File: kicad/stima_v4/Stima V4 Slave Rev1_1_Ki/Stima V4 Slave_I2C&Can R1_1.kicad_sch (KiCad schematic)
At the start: 45 parts, among them J2 6P, J3 3P, U4 TJA1443ATK, U5 NM PCA9616PW, U6 PCA9517D (TCA9517D), U7 ST732M50R, U8 AP22653QW6-7, U9 AP22653QW6-7

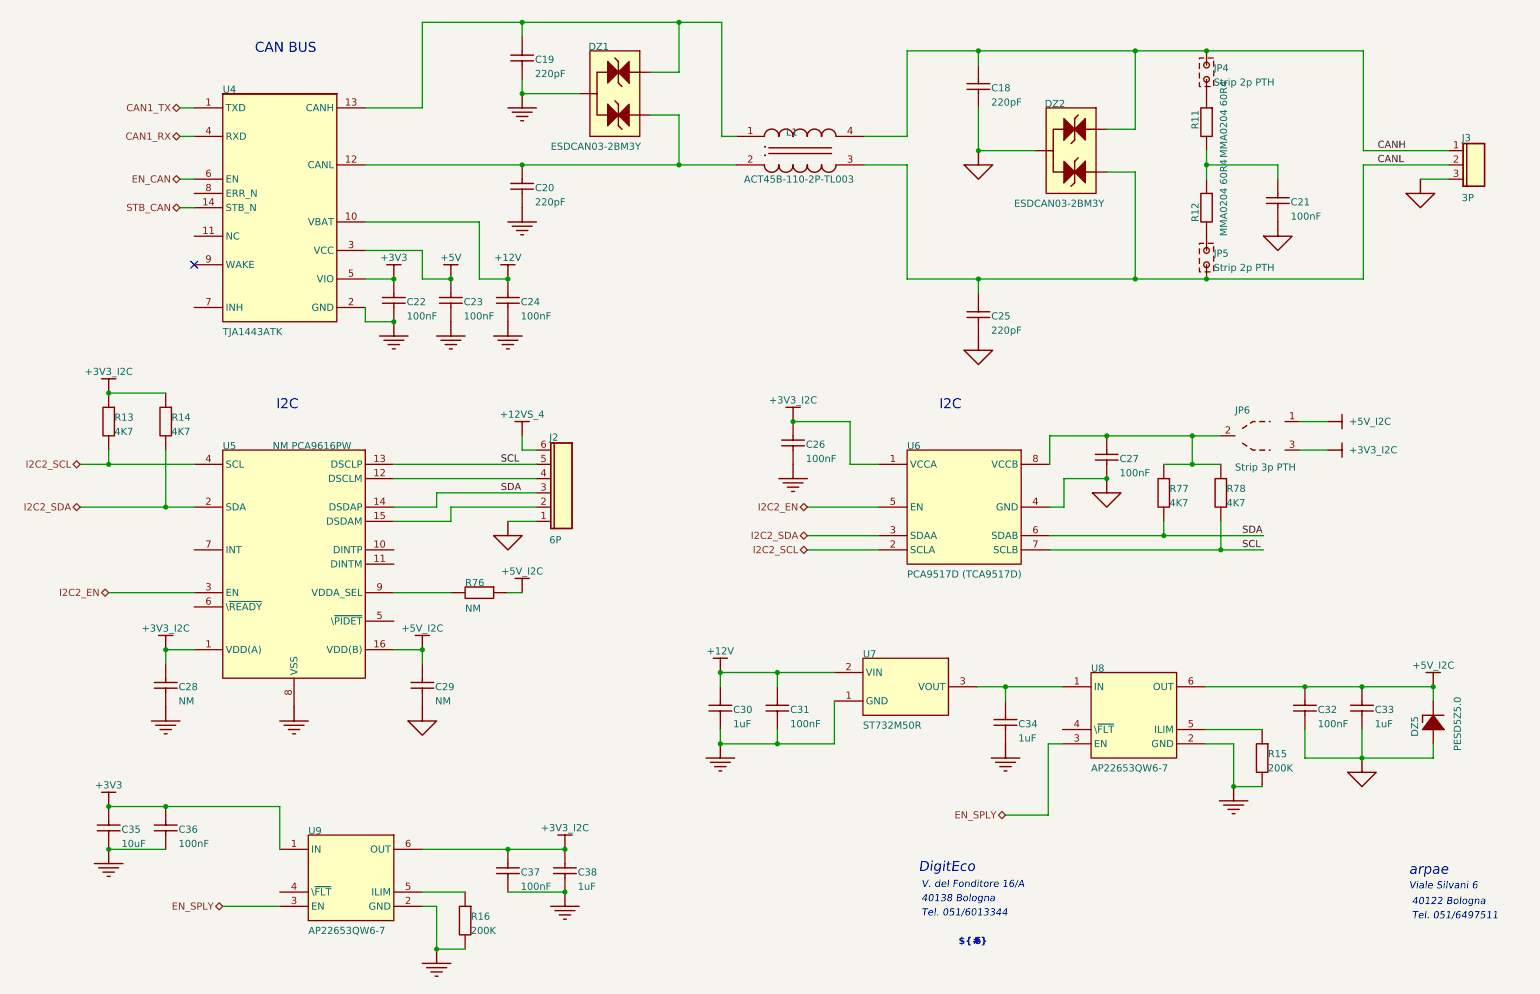
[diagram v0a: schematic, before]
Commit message: Update KiCad Stima V4
Add KiCad Stima V4 project
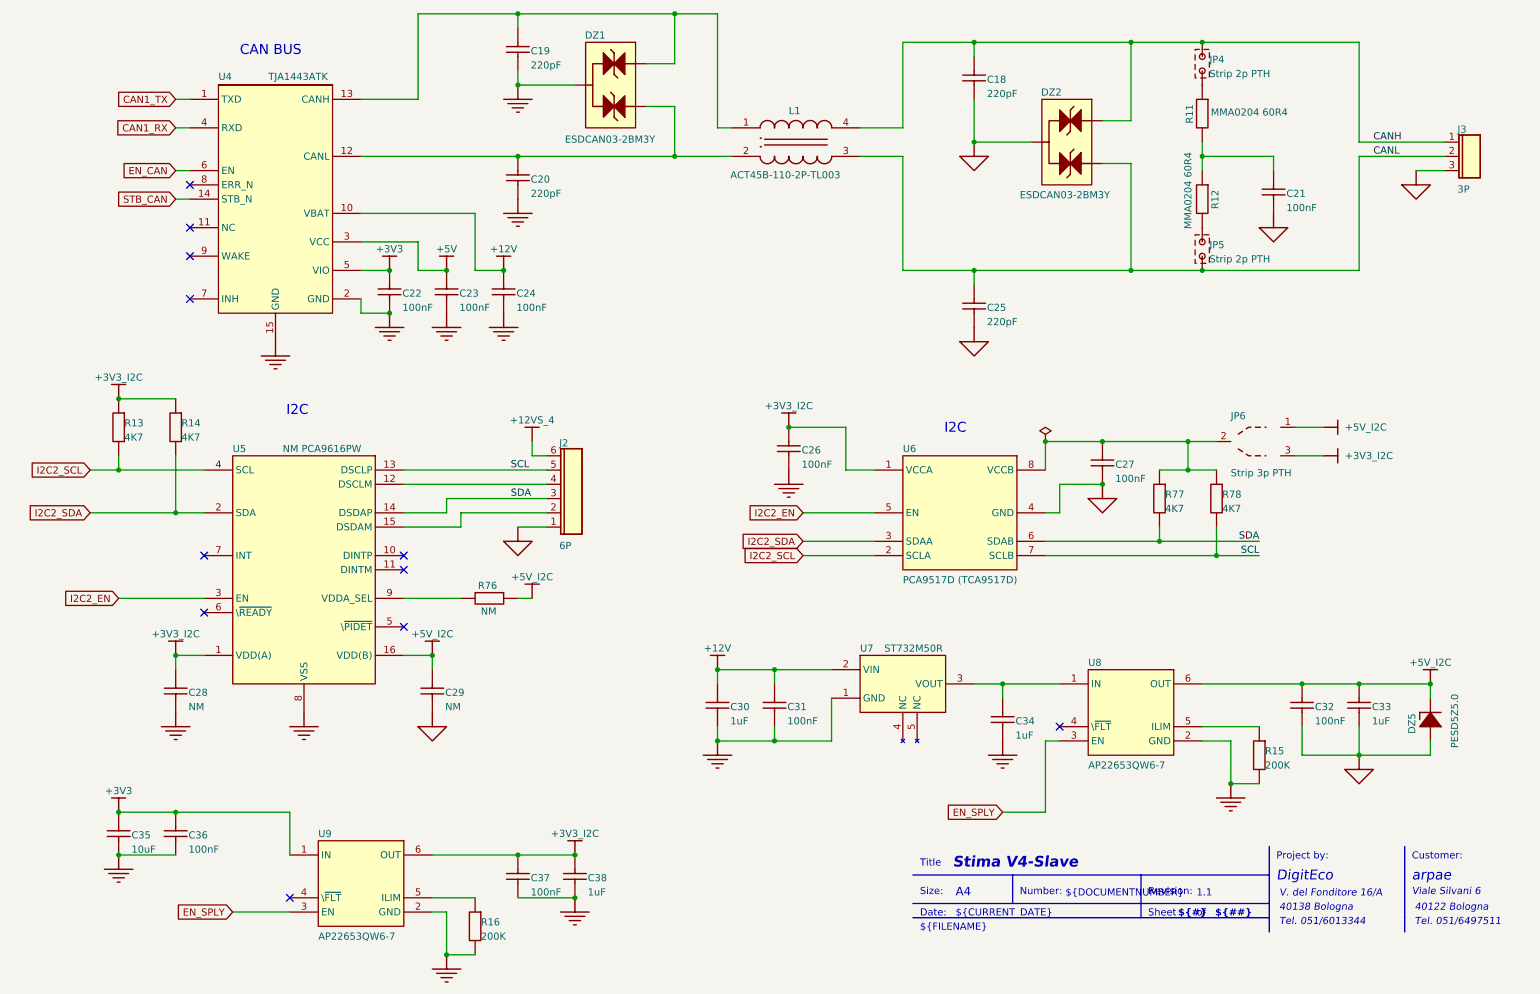
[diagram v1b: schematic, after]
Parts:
- C18, C19, C20, C21, C22, C23, C24, C25, C26, C27, C28, C29, C30, C31, C32, C33, C34, C35, C36, C37, C38, R13, R14, R15, R16, R76, R77, R78: footprint 0603 -> Library_Slave_impronte:0603
- DZ1, DZ2: footprint QFN-3L-DFN1110 -> Library_Slave_impronte:QFN-3L-DFN1110
- DZ5: footprint SOD 523(SC-79) -> Library_Slave_impronte:SOD 523(SC-79)
- J2: footprint CONN_6P-P381 -> Library_Slave_impronte:CONN_6P-P381
- J3: footprint CONN_3P-P381 -> Library_Slave_impronte:CONN_3P-P381
- JP4, JP5: footprint STRIP2P -> Library_Slave_impronte:STRIP2P
- JP6: footprint STRIP3PP254 -> Library_Slave_impronte:STRIP3PP254
- L1: footprint ACT45B TDK-MIO -> Library_Slave_impronte:ACT45B TDK-MIO
- R11, R12: footprint MELFRESMMA0204 -> Library_Slave_impronte:MELFRESMMA0204
- U4: footprint HVSON14 -> Library_Slave_impronte:HVSON14
- U5: footprint TSSOP16 -> Library_Slave_impronte:TSSOP16
- U6: footprint SO8 -> Library_Slave_impronte:SO8
- U7: footprint SOT23_5 -> Library_Slave_impronte:SOT23_5
- U8, U9: footprint SOT26 -> Library_Slave_impronte:SOT26
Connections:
- net GND: now also U4.15 (GND)
- no-connect marks 1 -> 11
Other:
- note added: "${##}"
- note added: "${CURRENT_DATE}"
- note added: "${DOCUMENTNUMBER}"
- note added: "${FILENAME}"
- note added: "${TITLE}"
- note added: "1.1"
- note added: "A4"
- note added: "Customer:"
- note added: "Date:"
- note added: "Number:"
- note added: "Project by:"
- note added: "Revision:"
- note added: "Sheet"
- note added: "Size:"
- note added: "Title"
- note added: "of"
- note removed: "6"
- moved on the sheet: C18, C19, C20, C21, C22, C23, C24, C25, C26, C27, C28, C29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
